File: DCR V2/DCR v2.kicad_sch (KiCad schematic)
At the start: 44 parts, among them J1 ANT, J10 TP3, J2 TP6, J3 LO, J4 PWR, J5 Audio, J6 TP1, J7 TP2, J8 TP5, J9 TP4, U1 BPF, U2 SA612, U3 78L06, U4 LM386

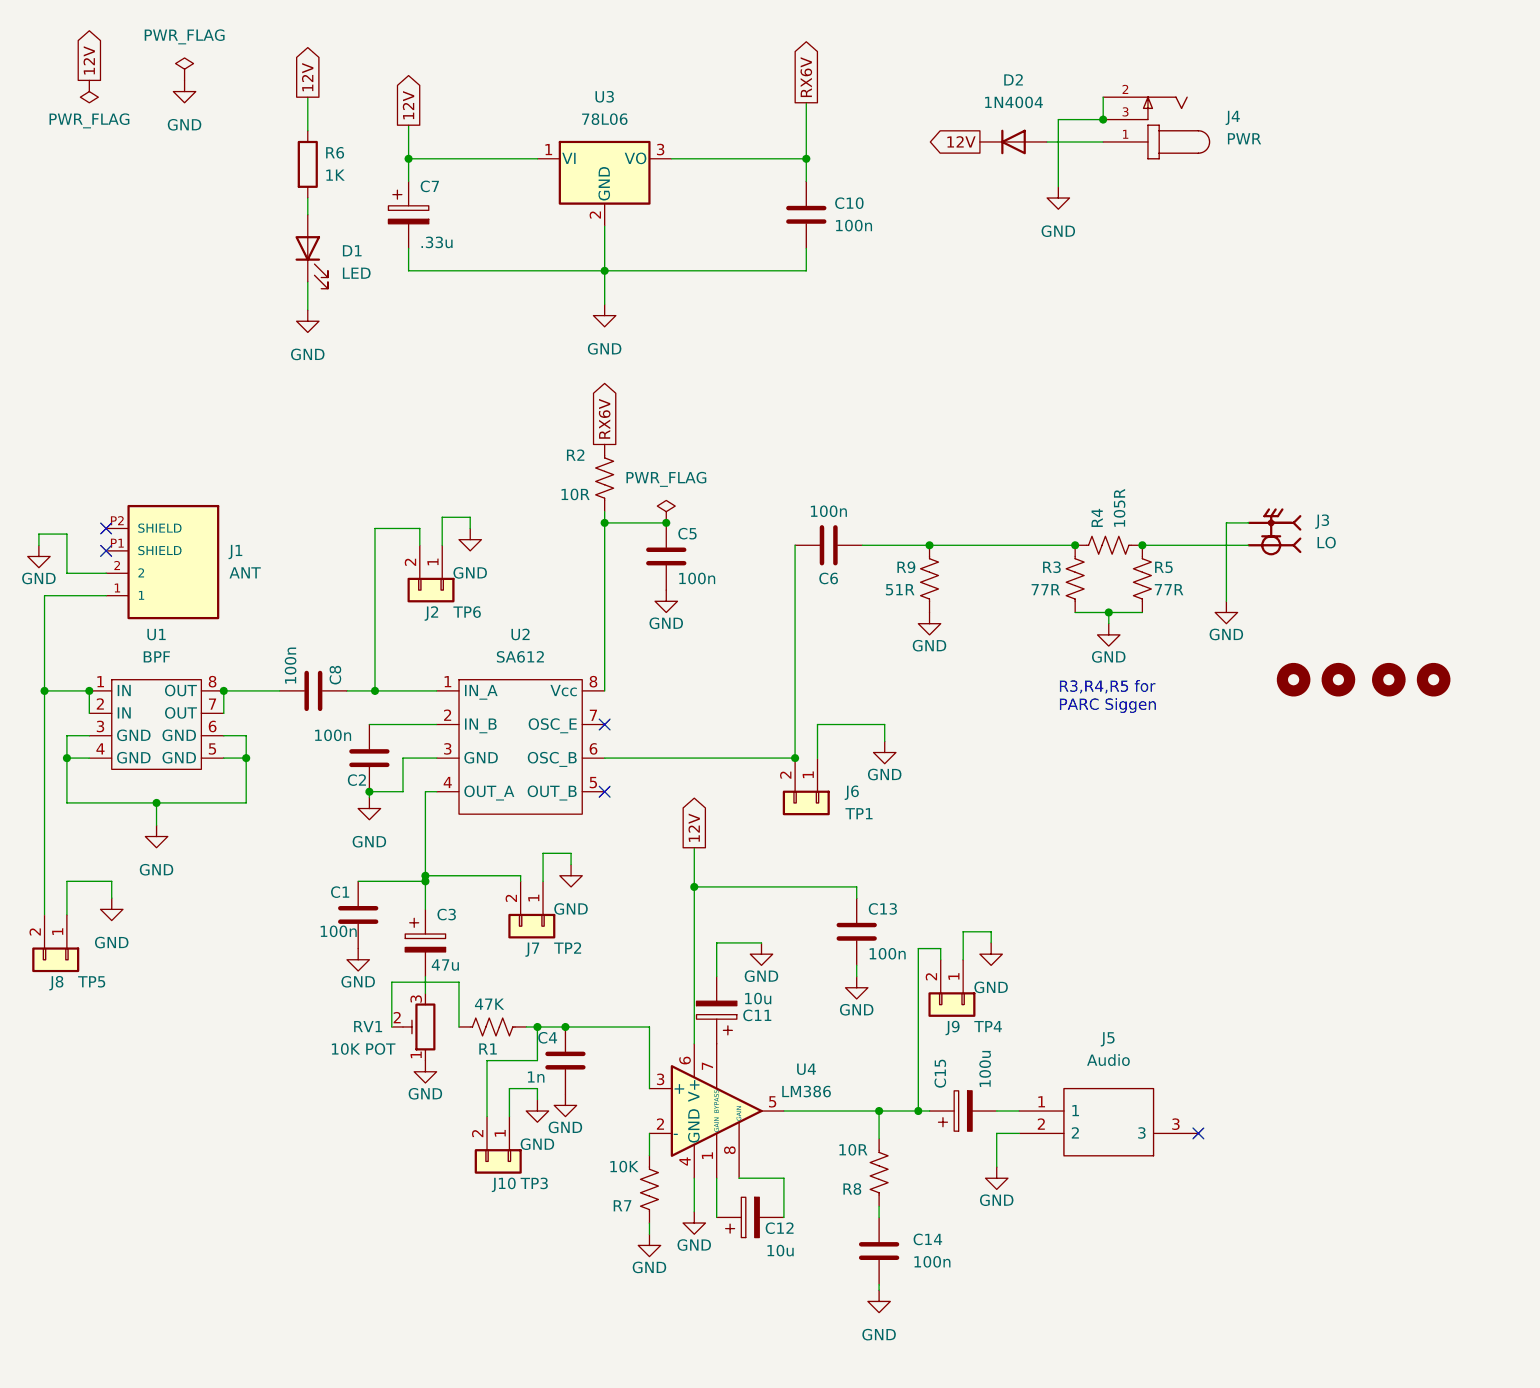
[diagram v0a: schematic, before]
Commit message: 7896 Update
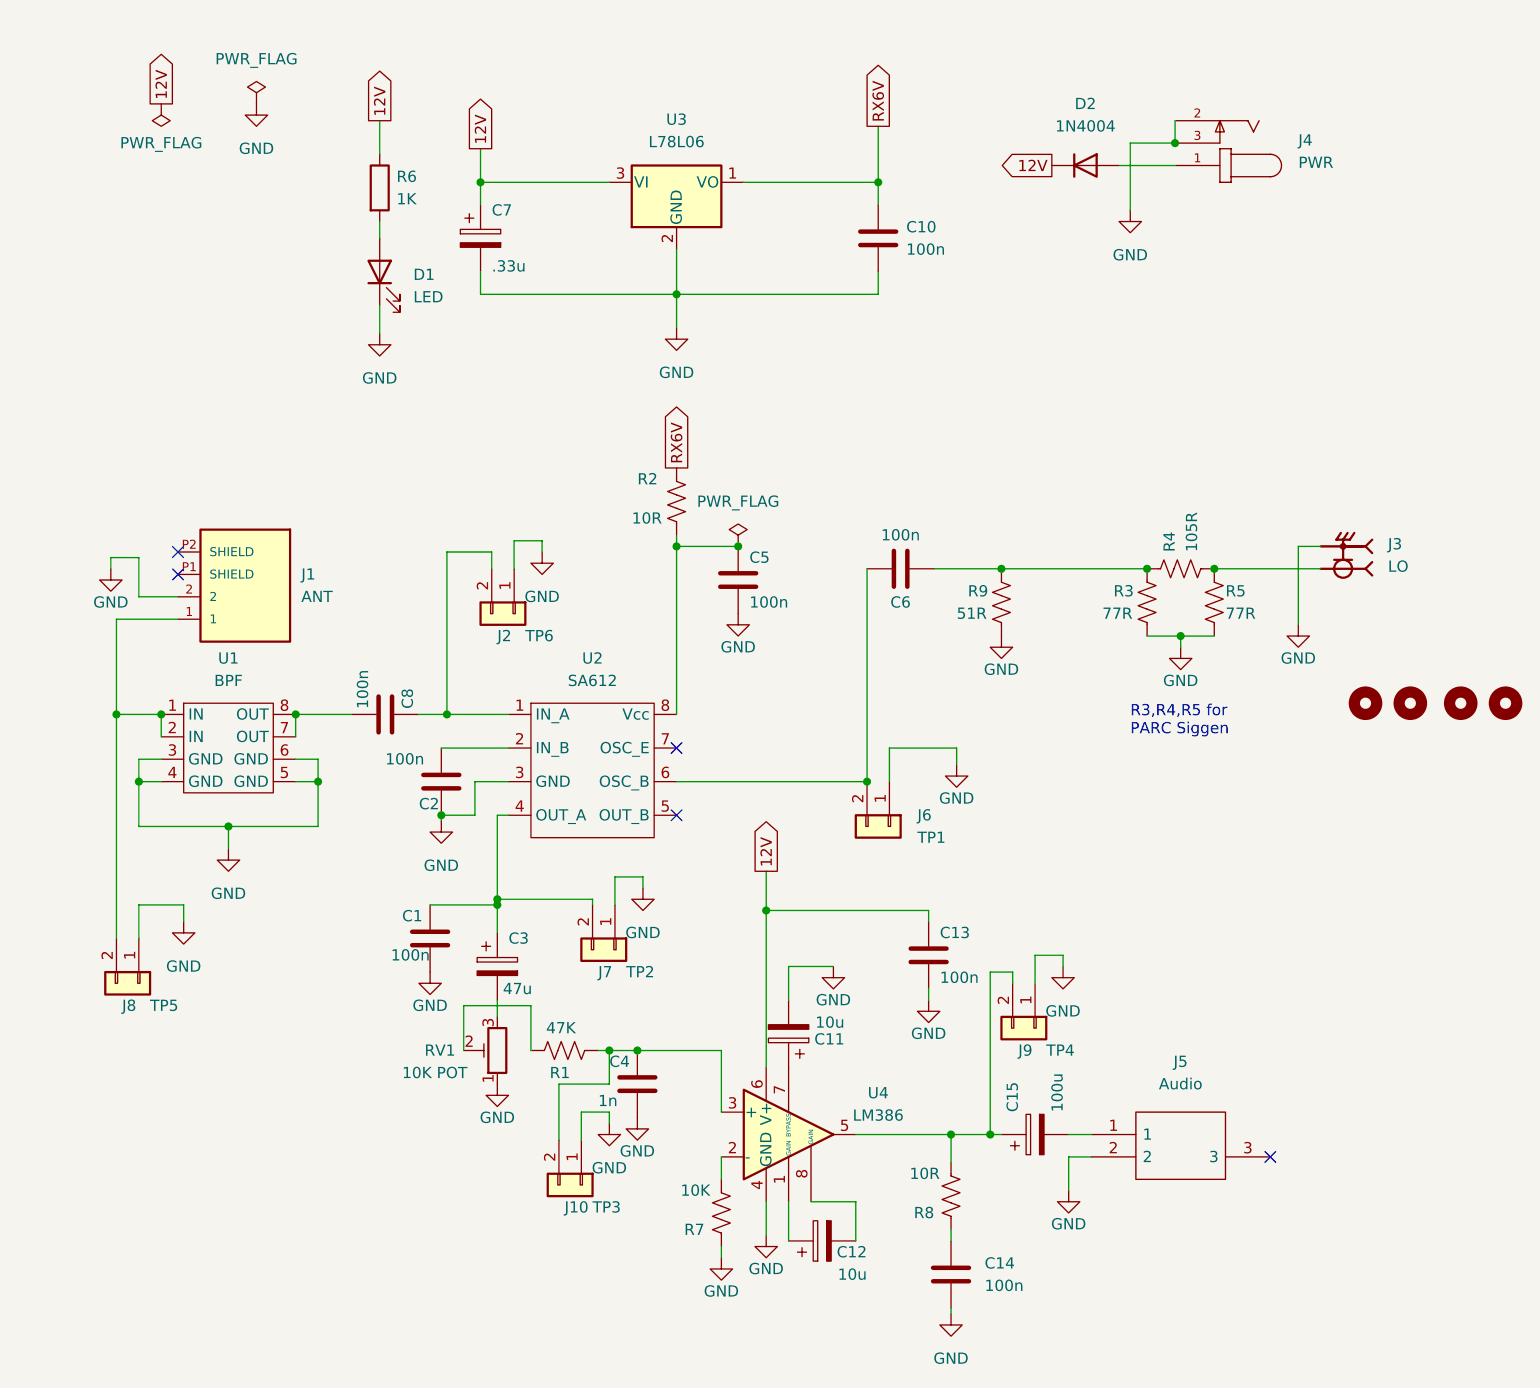
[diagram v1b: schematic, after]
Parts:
- removed U3: 78L06, Package_TO_SOT_THT:TO-92L_Inline_Wide, symbol Regulator_Linear:LM7805_TO220
- added U3: L78L06, Package_TO_SOT_THT:TO-92_Inline, symbol Regulator_Linear:L78L06_TO92
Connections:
- net 12V: now also U3.3 (VI)
- net GND: now also U3.2 (GND)
- net RX6V: now also U3.1 (VO)
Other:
- moved on the sheet: C1, C10, C11, C12, C13, C14, C15, C2, C3, C4, C5, C6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
